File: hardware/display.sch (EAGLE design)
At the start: 55 parts, among them IC5 7805DT

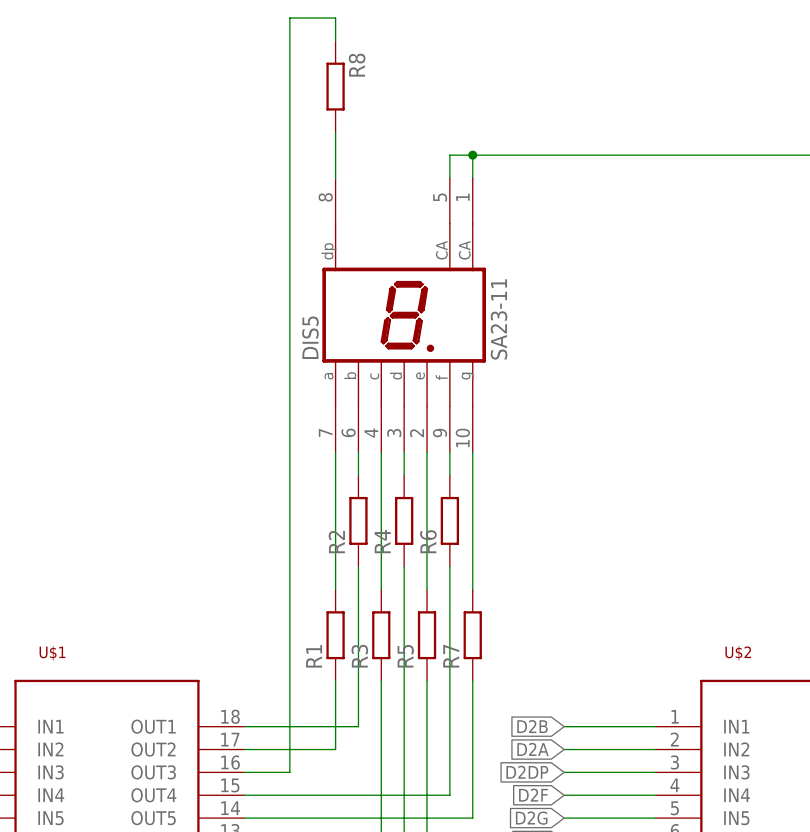
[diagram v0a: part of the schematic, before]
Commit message: Hardware project updates and fixes
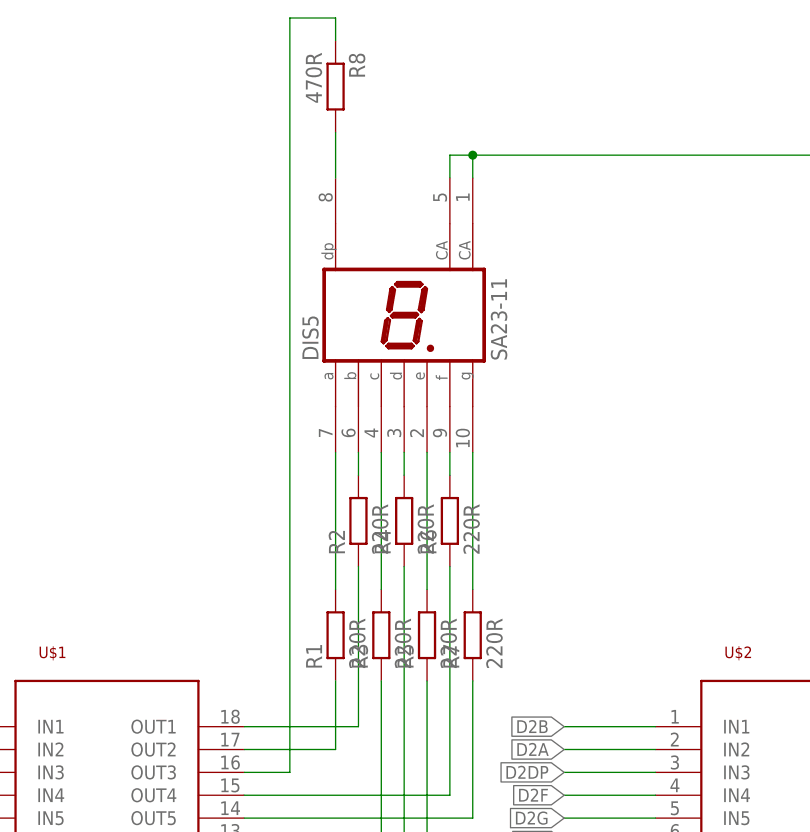
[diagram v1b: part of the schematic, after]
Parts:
- R1, R2, R3, R4, R5, R6, R7: value (none) -> 220R
- R8: value (none) -> 470R
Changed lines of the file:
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@@
 <part name="DIS2" library="display-kingbright" deviceset="SA23-11" device=""/>
 <part name="DIS3" library="display-kingbright" deviceset="SA23-11" device=""/>
-<part name="R1" library="rcl" deviceset="R-EU_" device="R0603"/>
-<part name="R2" library="rcl" deviceset="R-EU_" device="R0603"/>
-<part name="R3" library="rcl" deviceset="R-EU_" device="R0603"/>
-<part name="R4" library="rcl" deviceset="R-EU_" device="R0603"/>
-<part name="R5" library="rcl" deviceset="R-EU_" device="R0603"/>
-<part name="R6" library="rcl" deviceset="R-EU_" device="R0603"/>
-<part name="R7" library="rcl" deviceset="R-EU_" device="R0603"/>
-<part name="R8" library="rcl" deviceset="R-EU_" device="R0603"/>
+<part name="R1" library="rcl" deviceset="R-EU_" device="R0603" value="220R"/>
+<part name="R2" library="rcl" deviceset="R-EU_" device="R0603" value="220R"/>
+<part name="R3" library="rcl" deviceset="R-EU_" device="R0603" value="220R"/>
+<part name="R4" library="rcl" deviceset="R-EU_" device="R0603" value="220R"/>
+<part name="R5" library="rcl" deviceset="R-EU_" device="R0603" value="220R"/>
+<part name="R6" library="rcl" deviceset="R-EU_" device="R0603" value="220R"/>
+<part name="R7" library="rcl" deviceset="R-EU_" device="R0603" value="220R"/>
+<part name="R8" library="rcl" deviceset="R-EU_" device="R0603" value="470R"/>
 <part name="R9" library="rcl" deviceset="R-EU_" device="R0603"/>
 <part name="R10" library="rcl" deviceset="R-EU_" device="R0603"/>
